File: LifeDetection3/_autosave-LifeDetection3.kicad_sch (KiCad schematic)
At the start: 21 parts, among them J1 Power, J12 XT60PW-M, J2 PWM, J3 Analog, J4 PWM, J5 Analog, J6 Communication, J7 Digital, U1 TLP3545

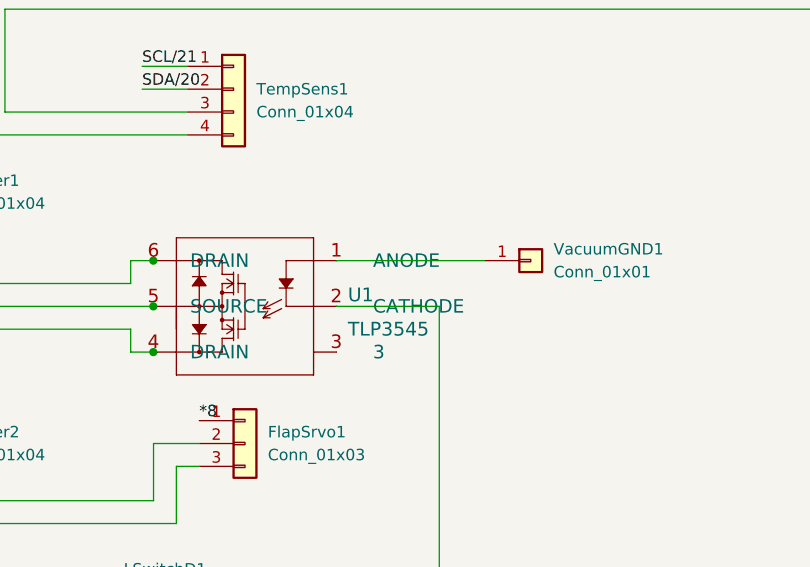
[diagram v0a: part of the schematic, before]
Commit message: almost done
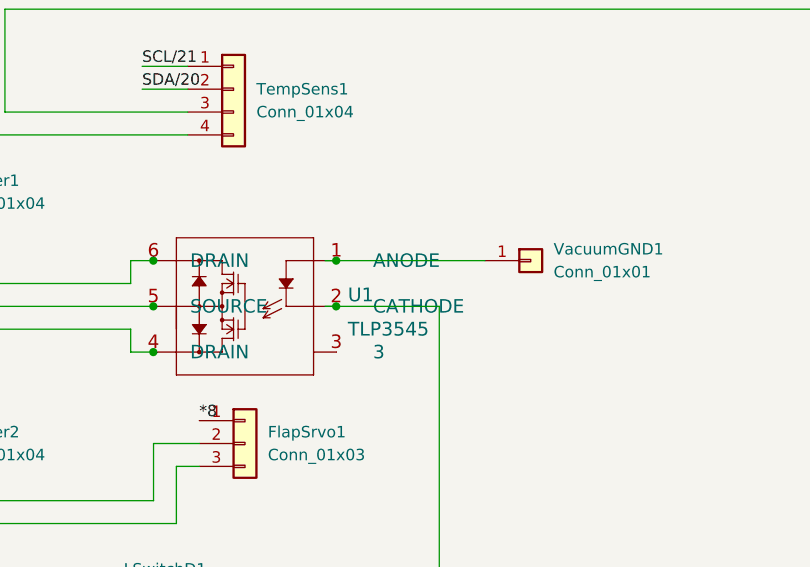
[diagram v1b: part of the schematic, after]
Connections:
- net at Dr1R1.1 (Pin_1), Dr2R1.1 (Pin_1), J12.2 (-): now also U1.2 (CATHODE)
- net at VacuumGND1.1 (Pin_1): now also U1.1 (ANODE)
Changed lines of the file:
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@@
     (date "mar. 31 mars 2015")
   )
+  (junction (at 143.4846 58.42) (diameter 0) (color 0 0 0 0)
+  )
   (junction (at 85.09 82.55) (diameter 0) (color 0 0 0 0)
   )
@@
   )
   (junction (at 85.09 54.61) (diameter 0) (color 0 0 0 0)
+  )
+  (junction (at 143.4846 53.34) (diameter 0) (color 0 0 0 0)
   )
   (junction (at 85.09 39.37) (diameter 0) (color 0 0 0 0)
@@
     (stroke (width 0) (type default) (color 0 0 0 0))
   )
+  (wire (pts (xy 143.4846 53.34) (xy 160.02 53.34))
+    (stroke (width 0) (type default) (color 0 0 0 0))
+  )
   (wire (pts (xy 57.15 44.45) (xy 92.71 44.45))
     (stroke (width 0) (type default) (color 0 0 0 0))
@@
     (stroke (width 0) (type default) (color 0 0 0 0))
   )
+  (wire (pts (xy 143.4846 58.42) (xy 154.94 58.42))
+    (stroke (width 0) (type default) (color 0 0 0 0))
+  )
   (wire (pts (xy 234.95 43.18) (xy 234.95 48.26))
     (stroke (width 0) (type solid) (color 0 0 0 0))
@@
     (stroke (width 0) (type solid) (color 0 0 0 0))
   )
-  (wire (pts (xy 143.51 53.34) (xy 160.02 53.34))
+  (wire (pts (xy 142.24 53.34) (xy 143.4846 53.34))
     (stroke (width 0) (type default) (color 0 0 0 0))
   )
@@
     (stroke (width 0) (type default) (color 0 0 0 0))
   )
+  (wire (pts (xy 142.24 58.42) (xy 143.4846 58.42))
+    (stroke (width 0) (type default) (color 0 0 0 0))
+  )
   (wire (pts (xy 265.43 66.04) (xy 278.13 66.04))
     (stroke (width 0) (type solid) (color 0 0 0 0))
@@
     (stroke (width 0) (type default) (color 0 0 0 0))
   )
-  (wire (pts (xy 143.51 58.42) (xy 154.94 58.42))
-    (stroke (width 0) (type default) (color 0 0 0 0))
-  )
